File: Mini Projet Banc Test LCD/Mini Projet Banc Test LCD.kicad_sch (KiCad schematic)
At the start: 8 parts

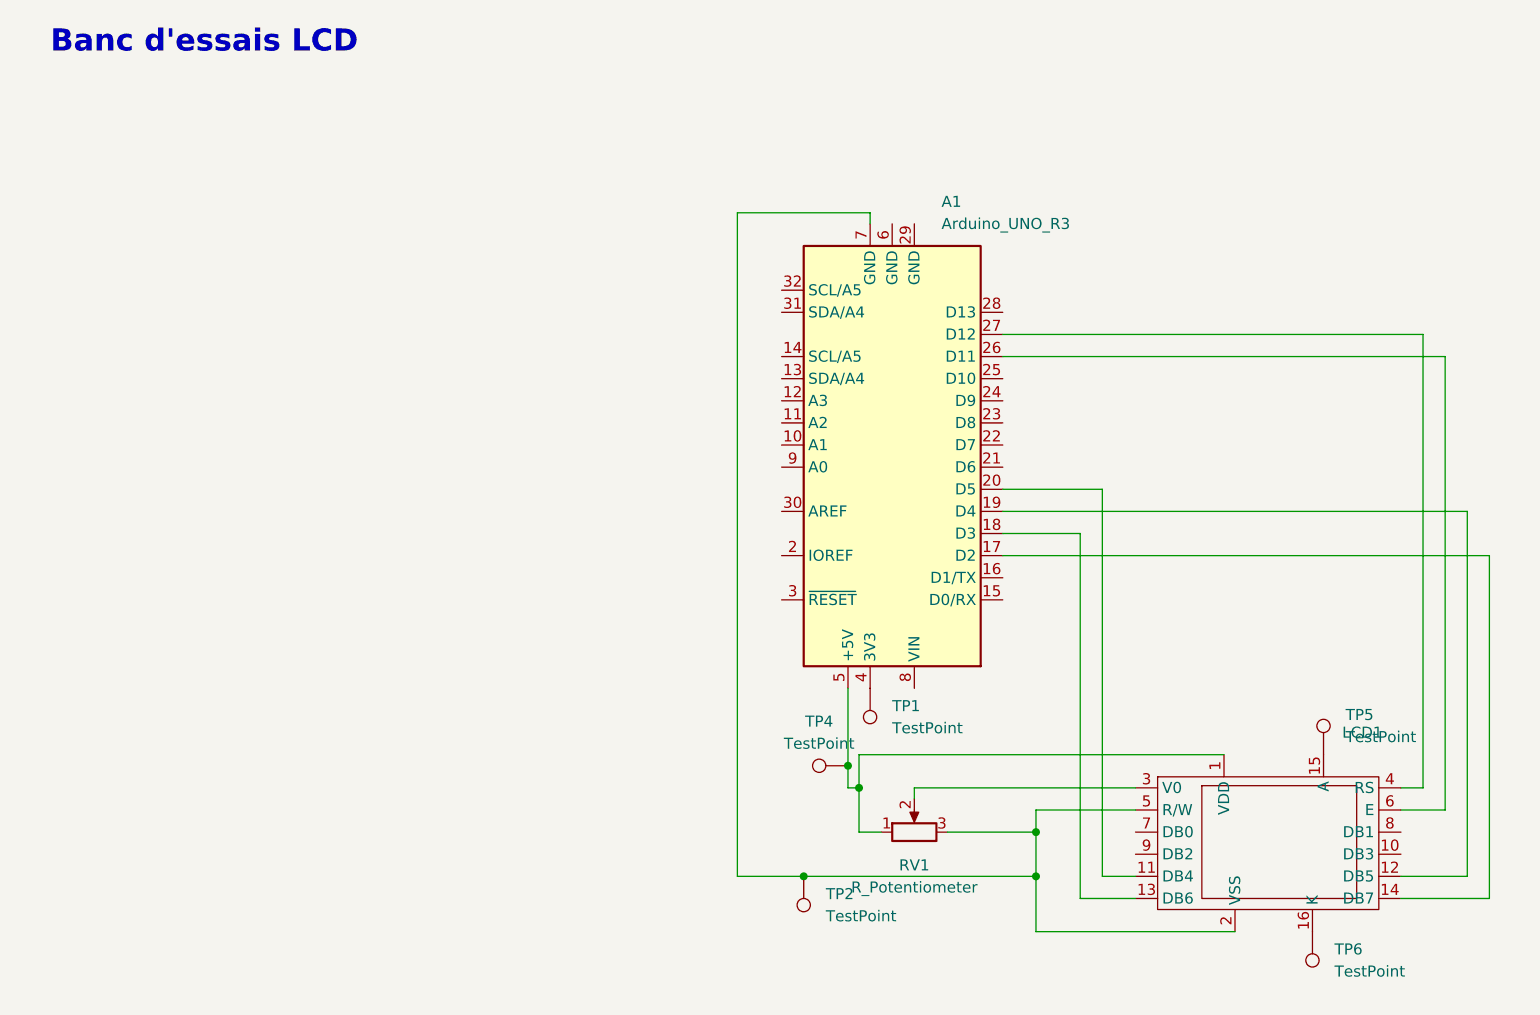
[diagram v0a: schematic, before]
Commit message: vendredi 02/12
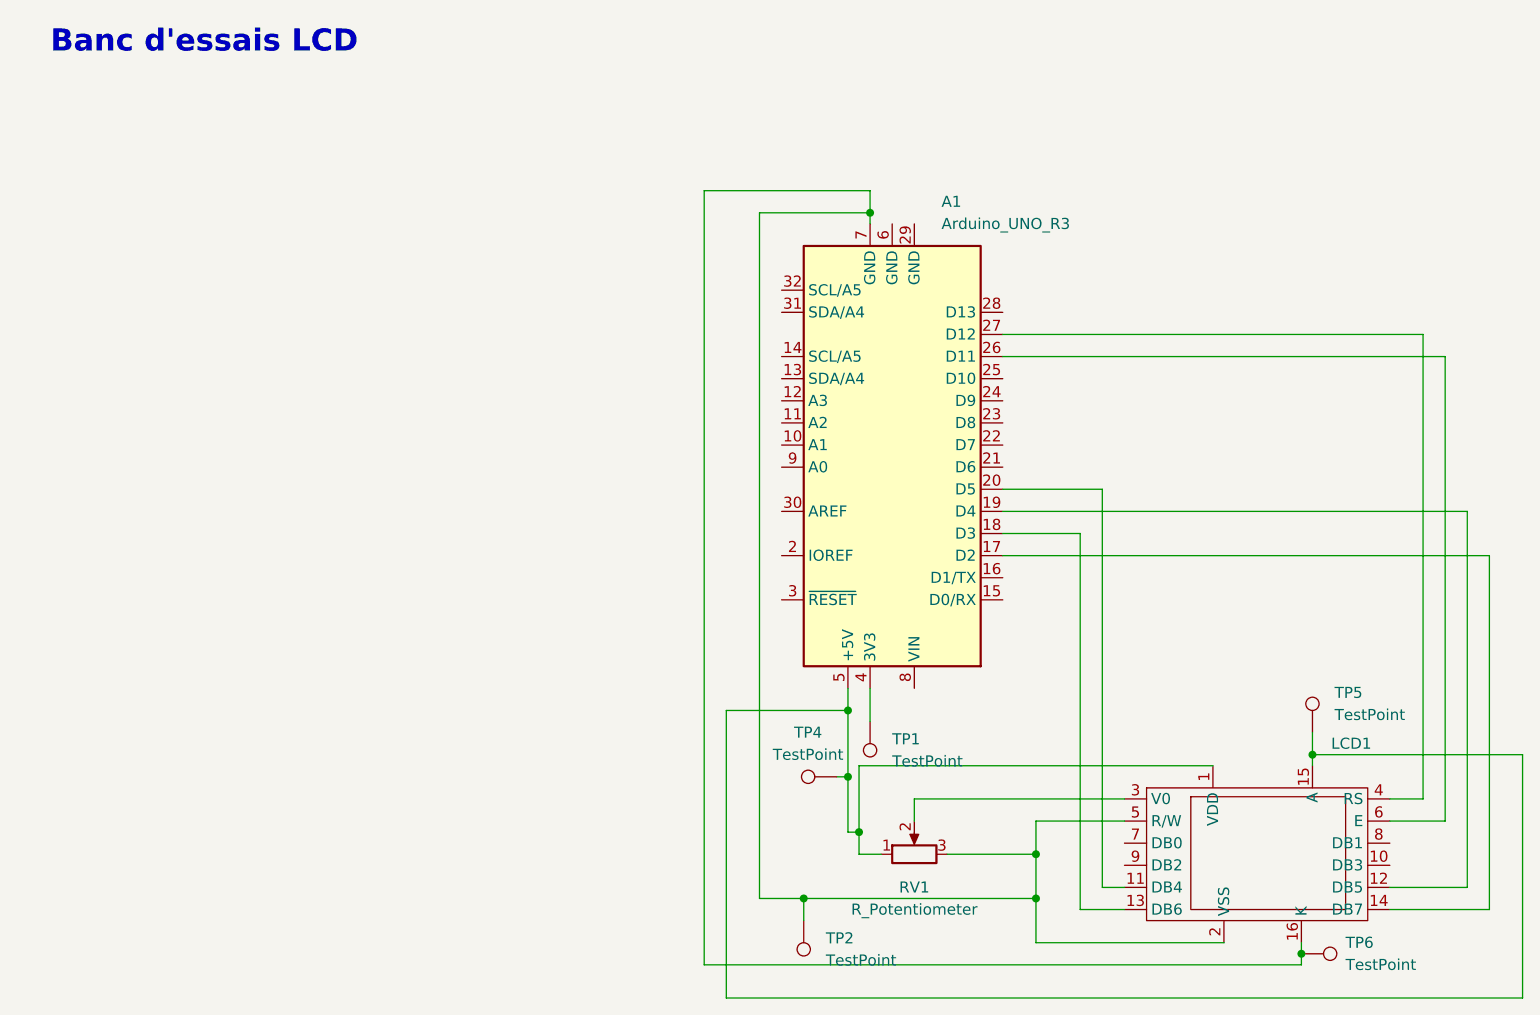
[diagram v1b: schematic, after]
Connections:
- net at A1.5 (+5V), LCD1.1 (VDD), RV1.1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: now also LCD1.15 (A), TP5.1
- net at A1.7 (GND), LCD1.2 (VSS), LCD1.5 (R/W)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: now also LCD1.16 (K), TP6.1
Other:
- moved on the sheet: LCD1, RV1, TP1, TP2, TP4, TP5, TP6
